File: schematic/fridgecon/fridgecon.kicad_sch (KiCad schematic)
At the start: 3 parts, among them J1 ICSPI, J2 MAX7219, U1 PIC12F675-xP

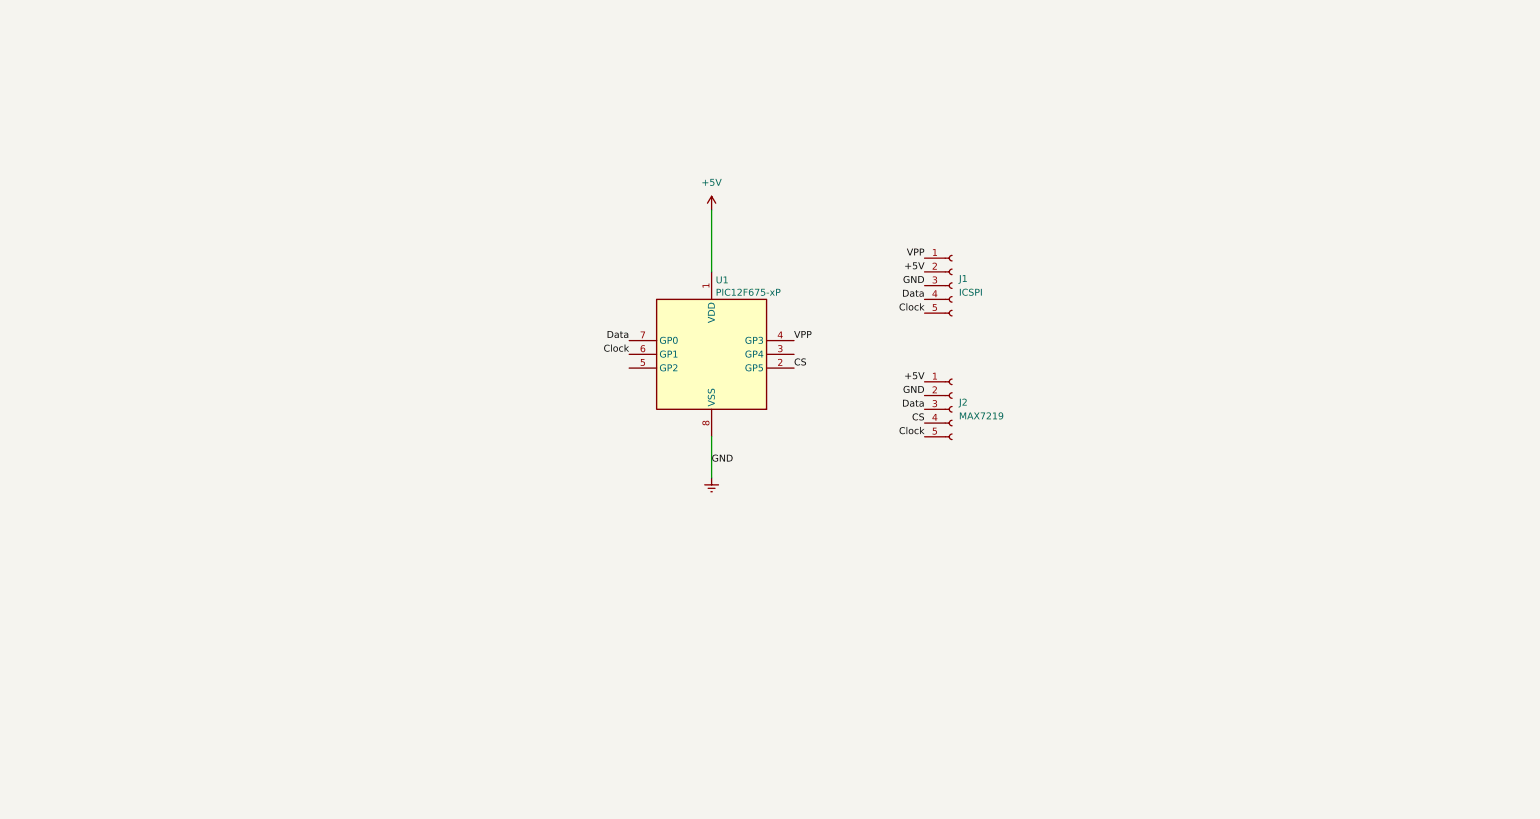
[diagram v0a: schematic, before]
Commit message: v1.0.0
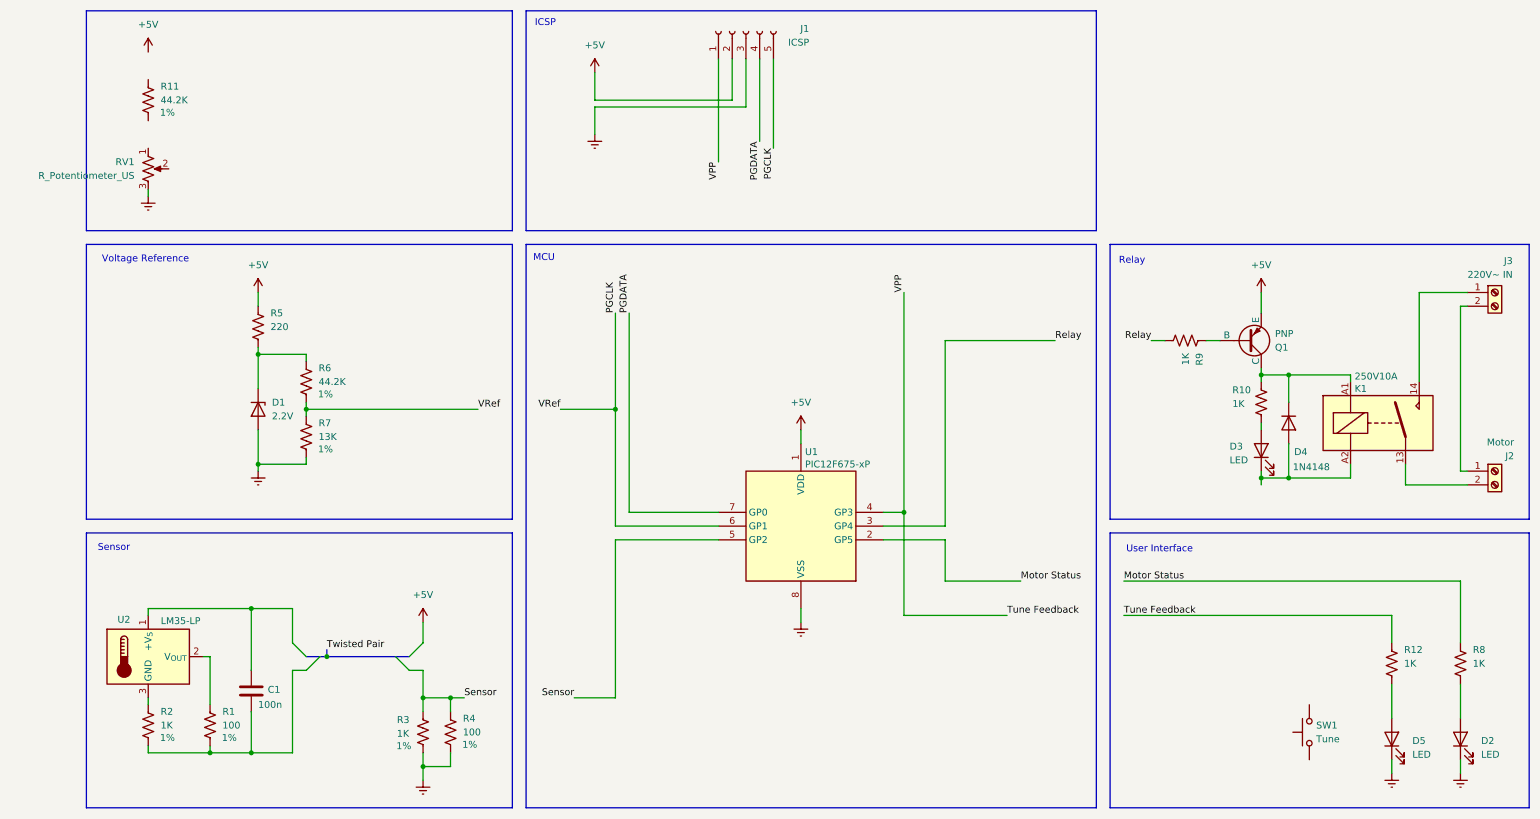
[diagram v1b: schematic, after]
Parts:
- removed J2: MAX7219, symbol Connector:Conn_01x05_Socket
- added C1: 100n, symbol Device:C
- added D1: 2.2V, symbol Device:D_Zener
- added D2, D3, D5: LED, symbol Device:LED
- added D4: 1N4148, Diode_THT:D_DO-35_SOD27_P7.62mm_Horizontal, symbol Diode:1N4148
- added J2: Motor, symbol Connector:Screw_Terminal_01x02
- added J3: 220V~ IN, symbol Connector:Screw_Terminal_01x02
- added K1: 250V10A, Relay_THT:Relay_SPST-NO_Fujitsu_FTR-LYAA005x_FormA_Vertical, symbol Relay:Fujitsu_FTR-LYAA005x
- added Q1: PNP, symbol Simulation_SPICE:PNP
- added R1, R4: 100, symbol Device:R_US
- added R10, R12, R2, R3, R8, R9: 1K, symbol Device:R_US
- added R11, R6: 44.2K, symbol Device:R_US
- added R5: 220, symbol Device:R_US
- added R7: 13K, symbol Device:R_US
- added RV1: R_Potentiometer_US, symbol Device:R_Potentiometer_US
- added SW1: Tune, symbol Switch:SW_Push
- added U2: LM35-LP, Package_TO_SOT_THT:TO-92_Inline, symbol Sensor_Temperature:LM35-LP
- J1: value ICSPI -> ICSP
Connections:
- net +5V: now also Q1.3 (E), R5.1
- net Relay: now reaches U1.3 (GP4)
- net Relay: now also R9.2
- net Sensor: now reaches U1.5 (GP2)
- net Sensor: now also R3.1, R4.1
- net CS renamed Motor Status
- net Motor Status: now also R8.1
- net Clock renamed PGCLK
- net PGCLK: now also R6.2, R7.1
- net Data renamed PGDATA
- net GND: no longer names the net of U1.8 (VSS)
- net GND: no longer J1.3 (Pin_3)
- net VPP renamed Tune Feedback
- net Tune Feedback: now also R12.1
- new net: D5.2 (A), R12.2
- new net: D1.1 (K), R5.2, R6.1
- new net: C1.1, U2.1 (+V_{S})
- new net: C1.2, R1.2, R2.2
- new net: Q1.2 (B), R9.1
- new net: D2.2 (A), R8.2
- new net: J2.2 (Pin_2), K1.13
- new net: J3.1 (Pin_1), K1.14
- new net: D4.1 (K), K1.A1, Q1.1 (C), R10.1
- new net: D3.1 (K), D4.2 (A), K1.A2
- new net: J2.1 (Pin_1), J3.2 (Pin_2)
- new net: D1.2 (A), R7.2
- new net: R3.2, R4.2
- new net: D3.2 (A), R10.2
- new net: R1.1, U2.2 (V_{OUT})
- new net: R2.1, U2.3 (GND)
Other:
- note added: "ICSP"
- note added: "MCU"
- note added: "Relay"
- note added: "Sensor"
- note added: "User Interface"
- note added: "Voltage Reference"
- moved on the sheet: U1
